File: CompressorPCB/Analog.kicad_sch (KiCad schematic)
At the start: 47 parts, among them Q1 NPN, Q2 PNP, Q3 PNP, U1 TL074, U2 TL074, U3 LM13700

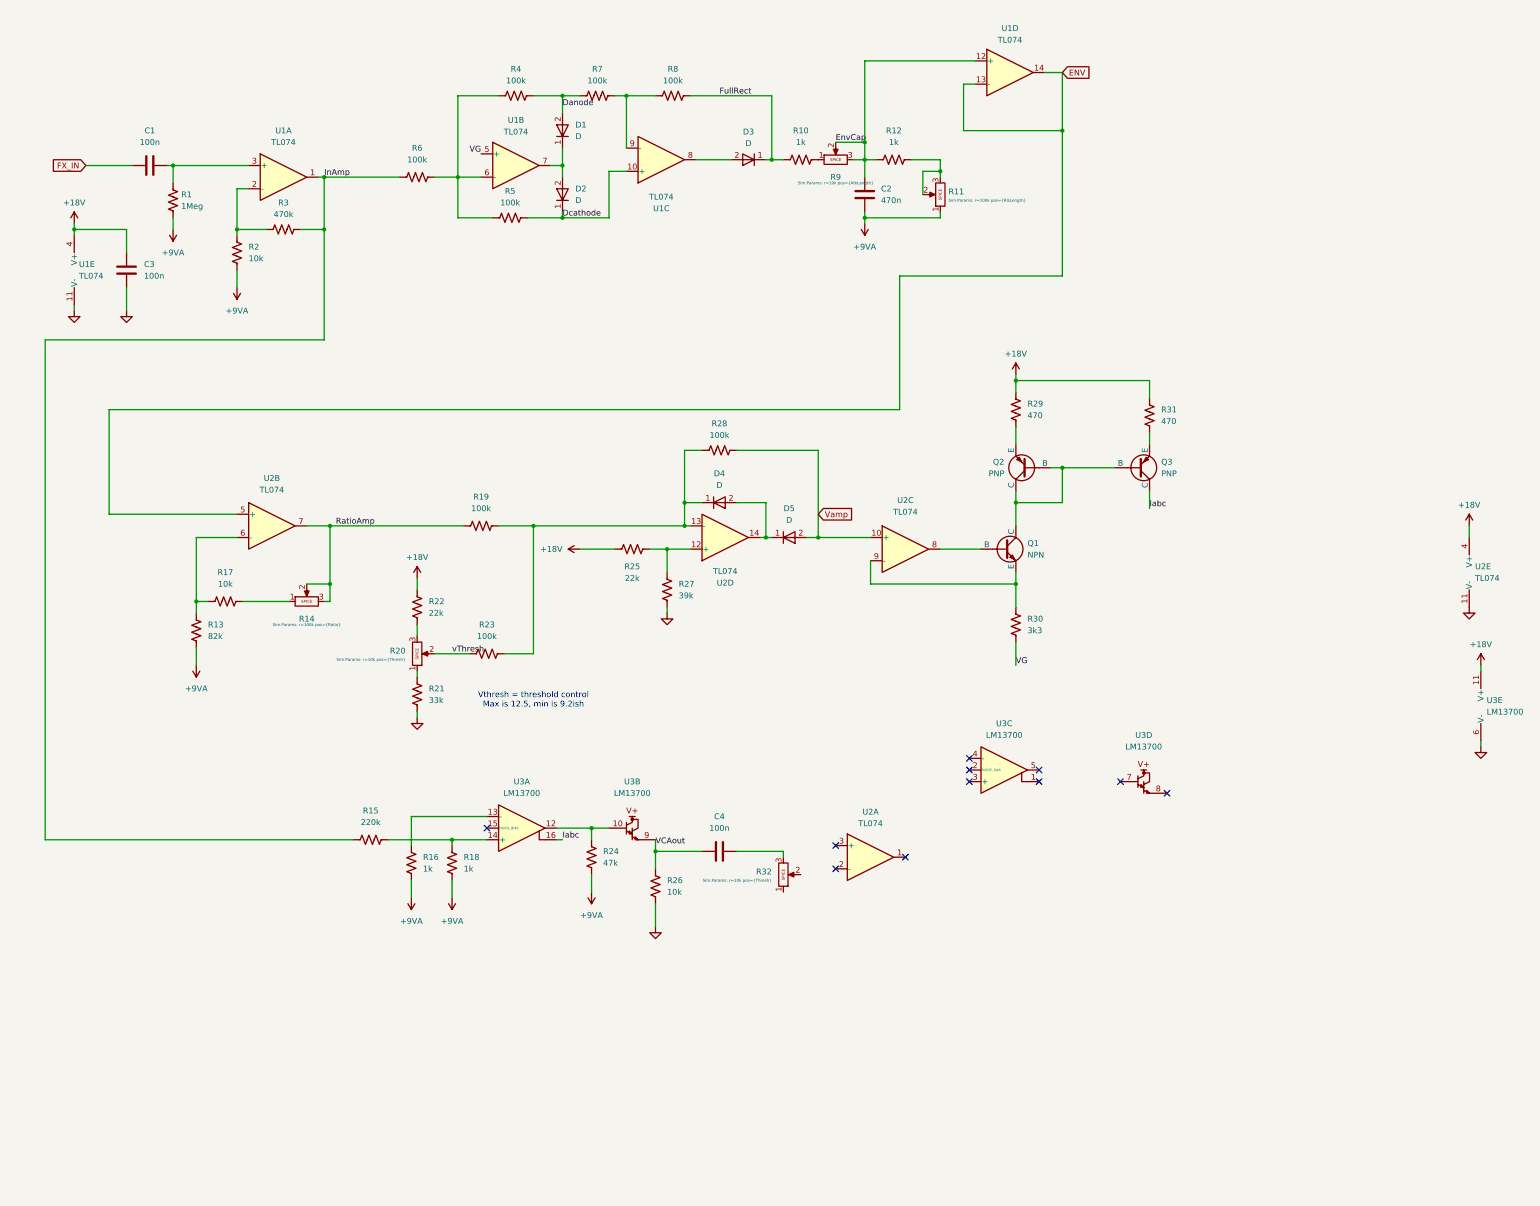
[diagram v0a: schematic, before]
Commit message: analog and power section schematics
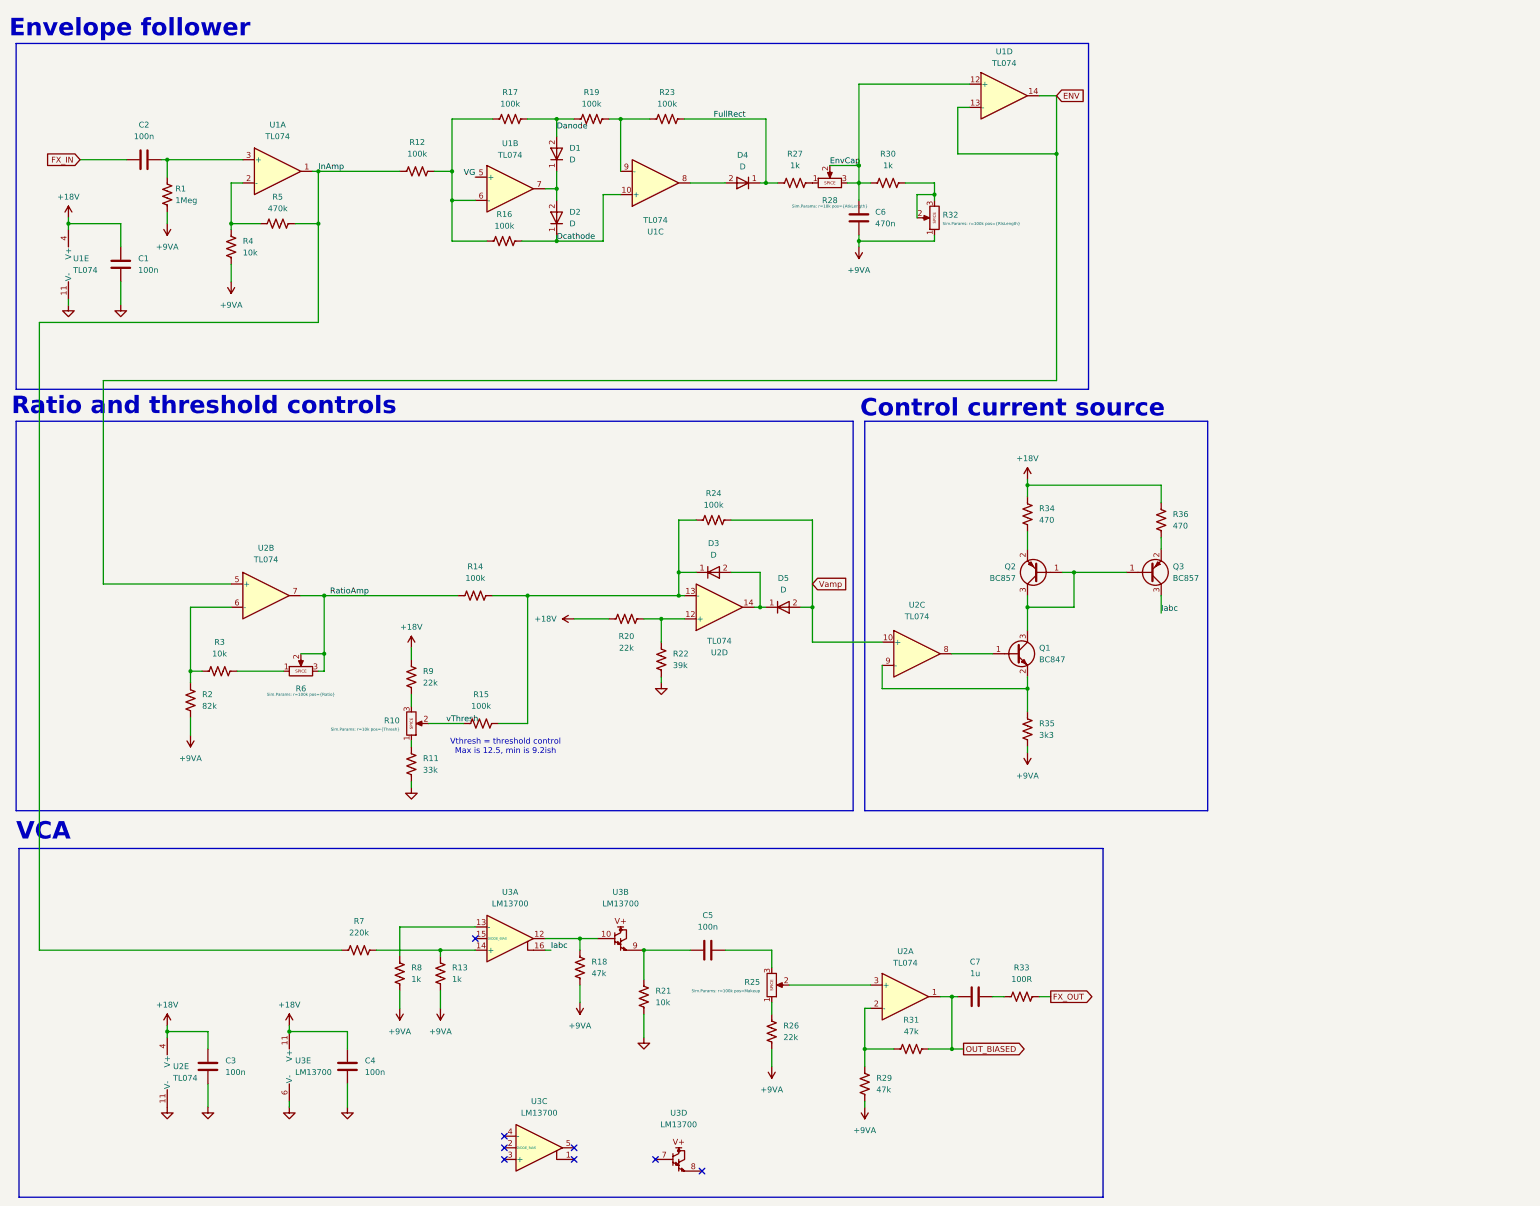
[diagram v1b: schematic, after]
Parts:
- removed Q1: NPN, symbol Simulation_SPICE:NPN
- removed Q2, Q3: PNP, symbol Simulation_SPICE:PNP
- added C3, C4: 100n, symbol Device:C
- added C7: 1u, symbol Device:C
- added Q1: BC847, Package_TO_SOT_SMD:SOT-23, symbol Transistor_BJT:BC847
- added Q2, Q3: BC857, Package_TO_SOT_SMD:SOT-23, symbol Transistor_BJT:BC857
- added R26: 22k, symbol Device:R_US
- added R29, R31: 47k, symbol Device:R_US
- added R33: 100R, symbol Device:R_US
- renumbered C3 to C1, C1 to C2, C4 to C5, C2 to C6, D4 to D3, D3 to D4, R20 to R10, R21 to R11, R6 to R12, R18 to R13, R19 to R14, R23 to R15, R5 to R16, R4 to R17, R24 to R18, R7 to R19, R13 to R2, R25 to R20, R26 to R21, R27 to R22, R8 to R23, R28 to R24, R32 to R25, R10 to R27, R9 to R28, R17 to R3, R12 to R30, R11 to R32, R29 to R34, R30 to R35, R31 to R36, R2 to R4, R3 to R5, R14 to R6, R15 to R7, R16 to R8, R22 to R9
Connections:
- net +18V: now also C3.2, C4.2
- net +9VA: now also R35.1, R26.2, R29.1
- net GND: now also C3.1, C4.1
- net Iabc: now also Q3.3 (C)
- net VG: no longer R35.1
- net at R25.1: now also R26.1
- net at R25.2: now also U2.3 (+)
- net at R36.1: now also Q3.2 (E)
- net at R34.1: now also Q2.2 (E)
- net at U2.8: now also Q1.1 (B)
- net at R35.2, U2.9 (-): now also Q1.2 (E)
- net OUT_BIASED: now reaches U2.1
- net OUT_BIASED: now also C7.1, R31.2
- net at U2.2 (-): now also R29.2, R31.1
- net VCAout: no longer names the net of C5.1, R21.1, U3.9
- new net: Q1.3 (C), Q2.1 (B), Q2.3 (C), Q3.1 (B)
- new net: C7.2, R33.1
- new net FX_OUT: R33.2
- no-connect marks 11 -> 8
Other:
- note added: "Control current source"
- note added: "Envelope follower"
- note added: "Ratio and threshold controls"
- note added: "VCA"
- moved on the sheet: C1, C2, C5, C6, D1, D2, D3, D4, D5, R1, R10, R11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
